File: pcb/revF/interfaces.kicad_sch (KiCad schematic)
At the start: 52 parts, among them CON7 SOUND, CON8 VGA, J5 TAPE IN, J6 TAPE OUT, J7 USB C, U18 ESP-12E, U19 AMS1117-3.3, U20 LM311, U21 UDA1334ATS

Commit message: RevF pcb
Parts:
- U21: footprint Package_SO:SSOP-16_4.4x5.2mm_P0.65mm -> footprints:SSOP-16_4.4x5.2mm_P0.65mm-extended
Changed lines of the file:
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@@
 			)
 		)
-		(property "Footprint" "Package_SO:SSOP-16_4.4x5.2mm_P0.65mm"
+		(property "Footprint" "footprints:SSOP-16_4.4x5.2mm_P0.65mm-extended"
 			(at 140.97 48.26 0)
 			(effects

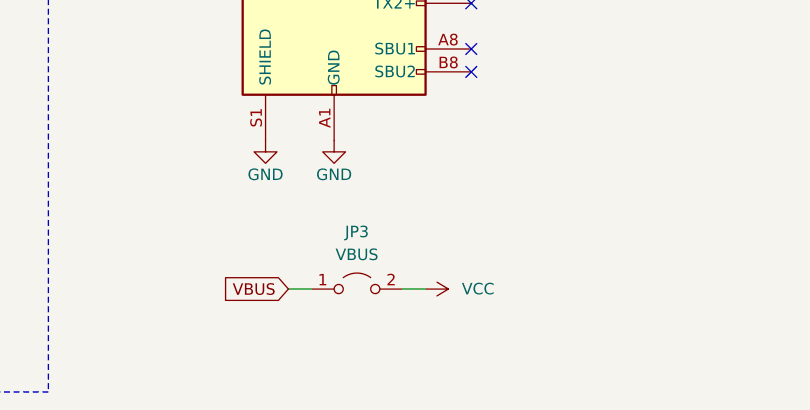
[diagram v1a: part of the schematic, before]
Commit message: Refactored revF alpha2
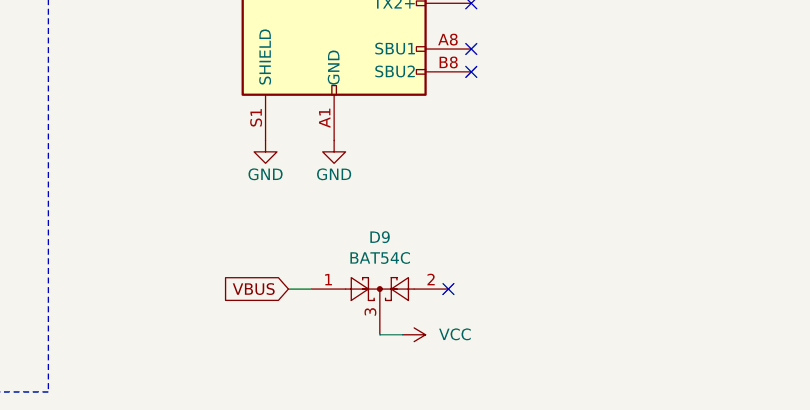
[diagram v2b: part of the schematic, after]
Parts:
- removed JP3: VBUS, Connector_PinHeader_2.54mm:PinHeader_1x02_P2.54mm_Vertical, symbol Jumper:Jumper_2_Open
- added D9: BAT54C, Package_TO_SOT_SMD:SOT-23_Handsoldering, symbol Diode:BAT54C
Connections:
- net VBUS: now also D9.1
- net VCC: now also D9.3
- no-connect marks 31 -> 32
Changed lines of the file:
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@@
 	)
 	(no_connect
+		(at 153.67 180.34)
+	)
+	(no_connect
 		(at 44.45 69.85)
 	)
@@
 	(wire
 		(pts
-			(xy 148.59 180.34) (xy 151.13 180.34)
+			(xy 146.05 185.42) (xy 148.59 185.42)
 		)
 		(stroke
@@
 	)
 	(symbol
-		(lib_id "Jumper:Jumper_2_Open")
-		(at 143.51 180.34 0)
-		(unit 1)
-		(exclude_from_sim no)
-		(in_bom yes)
-		(on_board yes)
-		(dnp no)
-		(fields_autoplaced yes)
-		(property "Reference" "JP3"
-			(at 143.51 173.99 0)
-			(effects
-				(font
-					(size 1.27 1.27)
-				)
-			)
-		)
-		(property "Value" "VBUS"
-			(at 143.51 176.53 0)
-			(effects
-				(font
-					(size 1.27 1.27)
-				)
-			)
-		)
-		(property "Footprint" "Connector_PinHeader_2.54mm:PinHeader_1x02_P2.54mm_Vertical"
-			(at 143.51 180.34 0)
-			(effects
-				(font
-					(size 1.27 1.27)
-				)
-				(hide yes)
-			)
-		)
-		(property "Datasheet" "~"
-			(at 143.51 180.34 0)
-			(effects
-				(font
-					(size 1.27 1.27)
-				)
-				(hide yes)
-			)
-		)
-		(property "Description" ""
-			(at 143.51 180.34 0)
-			(effects
-				(font
-					(size 1.27 1.27)
-				)
-			)
-		)
-		(pin "1"
-		)
-		(pin "2"
-		)
-		(instances
-			(project "karabas-pro-revF"
-				(path "/0fa36eda-2d7d-4199-a7a1-2cda6b0cd120/7f4e7edd-196d-4c95-a36b-79063a0e6ab2"
-					(reference "JP3")
-					(unit 1)
-				)
-			)
-		)
-	)
-	(symbol
 		(lib_id "Device:R")
 		(at 163.83 115.57 90)
@@
 	(symbol
 		(lib_id "power:VCC")
-		(at 151.13 180.34 270)
+		(at 148.59 185.42 270)
 		(unit 1)
 		(exclude_from_sim no)
@@
 		(dnp no)
 		(property "Reference" "#PWR034"
-			(at 147.32 180.34 0)
+			(at 144.78 185.42 0)
 			(effects
 				(font
@@
 		)
 		(property "Value" "VCC"
-			(at 156.972 180.34 90)
+			(at 154.432 185.42 90)
 			(effects
 				(font
@@
 		)
 		(property "Footprint" ""
-			(at 151.13 180.34 0)
+			(at 148.59 185.42 0)
 			(effects
 				(font
@@
 		)
 		(property "Datasheet" ""
-			(at 151.13 180.34 0)
+			(at 148.59 185.42 0)
 			(effects
 				(font
@@
 		)
 		(property "Description" ""
-			(at 151.13 180.34 0)
+			(at 148.59 185.42 0)
 			(effects
 				(font
@@
 					(unit 1)
 				)
+			)
+		)
+	)
+	(symbol
+		(lib_id "Diode:BAT54C")
+		(at 146.05 180.34 0)
+		(unit 1)
+		(exclude_from_sim no)
+		(in_bom yes)
+		(on_board yes)
+		(dnp no)
+		(property "Reference" "D9"
+			(at 146.05 174.625 0)
+			(effects
+				(font
+					(size 1.27 1.27)
+				)
+			)
+		)
+		(property "Value" "BAT54C"
+			(at 146.05 176.9364 0)
+			(effects
+				(font
+					(size 1.27 1.27)
+				)
+			)
+		)
+		(property "Footprint" "Package_TO_SOT_SMD:SOT-23_Handsoldering"
+			(at 147.955 177.165 0)
+			(effects
+				(font
+					(size 1.27 1.27)
+				)
+				(justify left)
+				(hide yes)
+			)
+		)
+		(property "Datasheet" "http://www.diodes.com/_files/datasheets/ds11005.pdf"
+			(at 144.018 180.34 0)
+			(effects
+				(font
+					(size 1.27 1.27)
+				)
+				(hide yes)
+			)
+		)
+		(property "Description" ""
+			(at 146.05 180.34 0)
+			(effects
+				(font
+					(size 1.27 1.27)
+				)
+			)
+		)
+		(pin "1"
+		)
+		(pin "2"
+		)
+		(pin "3"
+		)
+		(instances
+			(project "karabas-pro-revF"
+				(path "/0fa36eda-2d7d-4199-a7a1-2cda6b0cd120/7f4e7edd-196d-4c95-a36b-79063a0e6ab2"
+					(reference "D9")
+					(unit 1)
+				)
